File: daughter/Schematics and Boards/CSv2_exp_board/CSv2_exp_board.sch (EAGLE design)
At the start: 144 parts, among them J1 HIROSE-DF40_44-PIN_CONNECTORS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, J2 J-SERIAL-PORT, J3 CORTEX_DEBUG_SMD, J4 SJ-43514-SMT, J5 HIROSE-DF40_44-PIN_CONNECTORS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, J6 ATTINY_AVR_DEBUG, J7 J-USB-HIROSE-MICRO-USB, SW1 SPST_TACT-KMR2, SW2 SPST_TACT-KMR2, T1 TPTP10SQ, T10 TPTP10SQ, T11 TPTP10SQ, T2 TPTP10SQ, T3 TPTP10SQ, T4 TPTP10SQ, T5 TPTP10SQ, T6 TPTP10SQ, T7 TPTP10SQ, T8 TPTP10SQ, T9 TPTP10SQ, U1 LOADSWITCH-MIC94164, U10 LOADSWITCH-MIC94164, U11 BMI160, U12 TLV320DAC26IRHB, U13 ADG839YKSZ-500RL7KS_6_ADI-L, U14 LOADSWITCH-MIC94164, U15 LP2980AIM5-2.5/NOPBMF05A_TEX-L, U16 NCP553SQ18T1GSC-82AB_ONS-L, U17 ATTINY817-MFRQFN24_RX4MC-L_AT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, U18 MPL3115A2, U19 ATSAMD21G18_QFN, U2 ADA4841-1YRJZ-R7RJ_6-L, U3 Value, U4 RFM69HCW, U5 Value, U6 Value, U7 LOADSWITCH-MIC94164, U8 LOADSWITCH-MIC94164, U9 LOADSWITCH-MIC94164, X1 32.768kHz, X2 32.768, X3 uFL, X4 uFL, X5 uFL, X6 uFL

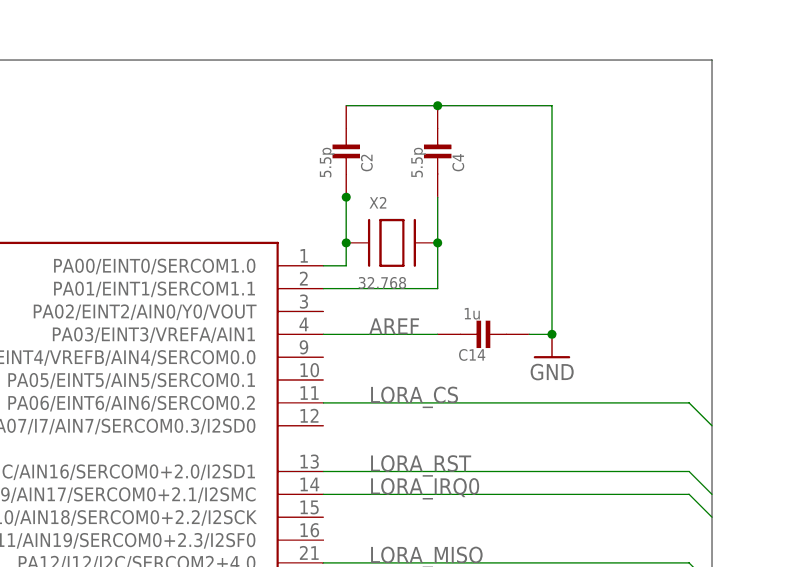
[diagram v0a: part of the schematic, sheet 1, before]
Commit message: DTR-filled in device attributes
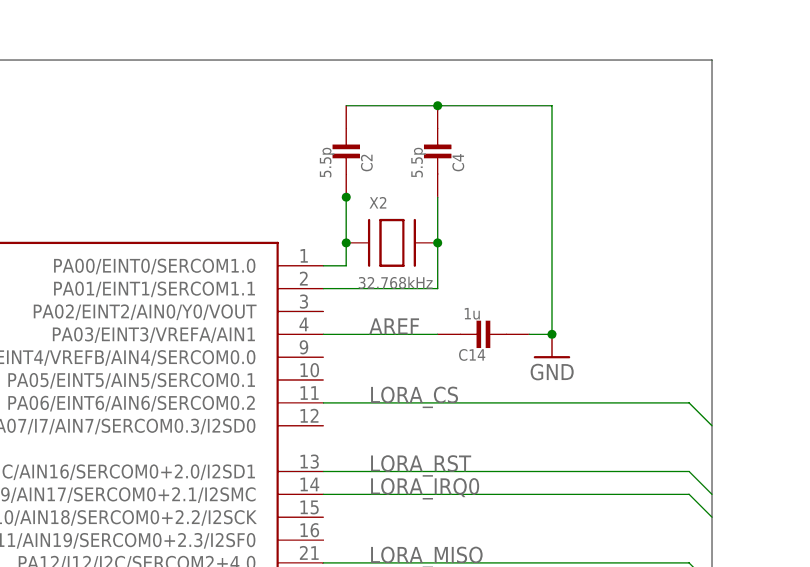
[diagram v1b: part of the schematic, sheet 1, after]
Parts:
- X2: value 32.768 -> 32.768kHz; DESC (none) -> CRYSTAL 32.7680KHZ 6PF SMD; HEIGHT (none) -> 0.9mm; LOAD_CAPACITY 6p -> 6pF; SIZE (none) -> 0.126" L x 0.059" W (3.20mm x 1.50mm); TOL (none) -> ±20ppm; TYPE (none) -> Crystal
- X3, X5, X6: DESC (none) -> CONN U.FL RCPT STR 50 OHM SMD; HEIGHT d -> 1.25mm; MANUFACTURER (none) -> Hirose; SIZE (none) -> 3.1 x 3mm; TYPE (none) -> Connector
- X4: DESC (none) -> CONN U.FL RCPT STR 50 OHM SMD; HEIGHT (none) -> 1.25mm; MEANUFACTURER (none) -> Hirose; SIZE (none) -> 3.1 x 3mm; TYPE (none) -> Connector
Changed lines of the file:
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@@
 <attribute name="Z-HEIGHT" value="0.55mm"/>
 </part>
-<part name="X2" library="CommonSense-DTR-v1" deviceset="ADAFRUIT2_XTAL" device="-3.2X1.5" value="32.768">
-<attribute name="DESC" value=""/>
-<attribute name="LOAD_CAPACITY" value="6p"/>
+<part name="X2" library="CommonSense-DTR-v1" deviceset="ADAFRUIT2_XTAL" device="-3.2X1.5" value="32.768kHz">
+<attribute name="DESC" value="CRYSTAL 32.7680KHZ 6PF SMD"/>
+<attribute name="HEIGHT" value="0.9mm"/>
+<attribute name="LOAD_CAPACITY" value="6pF"/>
 <attribute name="MANUFACTURER" value="NDK"/>
 <attribute name="MPN" value="NX3215SA-32.768K-STD-MUA-14"/>
 <attribute name="PARTNO" value="NX3215SA-32.768K-STD-MUA-14"/>
-<attribute name="SIZE" value=""/>
-<attribute name="TOL" value=""/>
-<attribute name="TYPE" value=""/>
-<attribute name="VOLT" value=""/>
+<attribute name="SIZE" value="0.126&quot; L x 0.059&quot; W (3.20mm x 1.50mm)"/>
+<attribute name="TOL" value="±20ppm"/>
+<attribute name="TYPE" value="Crystal"/>
 </part>
 <part name="U$14" library="Supplies" deviceset="GND" device=""/>
@@
 <part name="U$17" library="Supplies" deviceset="GND" device=""/>
 <part name="X4" library="Connectors" deviceset="J-U.FL" device="" value="uFL">
-<attribute name="DESC" value=""/>
+<attribute name="DESC" value="CONN U.FL RCPT STR 50 OHM SMD"/>
+<attribute name="HEIGHT" value="1.25mm"/>
+<attribute name="MEANUFACTURER" value="Hirose"/>
 <attribute name="MPN" value="U.FL-R-SMT-1(01)"/>
 <attribute name="PARTNO" value="U.FL-R-SMT-1(01)"/>
-<attribute name="SIZE" value=""/>
-<attribute name="TOL" value=""/>
-<attribute name="TYPE" value=""/>
-<attribute name="VOLT" value=""/>
+<attribute name="SIZE" value="3.1 x 3mm"/>
+<attribute name="TYPE" value="Connector"/>
 </part>
 <part name="U$23" library="Supplies" deviceset="GND" device=""/>
@@
 </part>
 <part name="X3" library="Connectors" deviceset="J-U.FL" device="" value="uFL">
-<attribute name="HEIGHT" value="d"/>
+<attribute name="DESC" value="CONN U.FL RCPT STR 50 OHM SMD"/>
+<attribute name="HEIGHT" value="1.25mm"/>
+<attribute name="MANUFACTURER" value="Hirose"/>
 <attribute name="MPN" value="U.FL-R-SMT-1(01)"/>
 <attribute name="PARTNO" value="U.FL-R-SMT-1(01)"/>
+<attribute name="SIZE" value="3.1 x 3mm"/>
+<attribute name="TYPE" value="Connector"/>
 </part>
 <part name="X5" library="Connectors" deviceset="J-U.FL" device="" value="uFL">
-<attribute name="HEIGHT" value="d"/>
+<attribute name="DESC" value="CONN U.FL RCPT STR 50 OHM SMD"/>
+<attribute name="HEIGHT" value="1.25mm"/>
+<attribute name="MANUFACTURER" value="Hirose"/>
 <attribute name="MPN" value="U.FL-R-SMT-1(01)"/>
 <attribute name="PARTNO" value="U.FL-R-SMT-1(01)"/>
+<attribute name="SIZE" value="3.1 x 3mm"/>
+<attribute name="TYPE" value="Connector"/>
 </part>
 <part name="X6" library="Connectors" deviceset="J-U.FL" device="" value="uFL">
-<attribute name="HEIGHT" value="d"/>
+<attribute name="DESC" value="CONN U.FL RCPT STR 50 OHM SMD"/>
+<attribute name="HEIGHT" value="1.25mm"/>
+<attribute name="MANUFACTURER" value="Hirose"/>
 <attribute name="MPN" value="U.FL-R-SMT-1(01)"/>
 <attribute name="PARTNO" value="U.FL-R-SMT-1(01)"/>
+<attribute name="SIZE" value="3.1 x 3mm"/>
+<attribute name="TYPE" value="Connector"/>
 </part>
 <part name="R7" library="Resistors" deviceset="R-" device="0402" value="50R">
@@
 <attribute name="TYPE" x="284.48" y="231.14" size="1.778" layer="96" display="off"/>
 <attribute name="SIZE" x="284.48" y="231.14" size="1.778" layer="96" display="off"/>
-<attribute name="VOLT" x="284.48" y="231.14" size="1.778" layer="96" display="off"/>
+<attribute name="HEIGHT" x="284.48" y="231.14" size="1.778" layer="96" display="off"/>
 </instance>
 <instance part="U$14" gate="1" x="101.6" y="233.68" smashed="yes">
@@
 <attribute name="MPN" x="78.62295625" y="212.957171875" size="1.778" layer="96" rot="R90" display="off"/>
 <attribute name="PARTNO" x="78.62295625" y="212.957171875" size="1.778" layer="96" display="off"/>
-<attribute name="TOL" x="78.62295625" y="212.957171875" size="1.778" layer="96" rot="R90" display="off"/>
 <attribute name="DESC" x="78.62295625" y="212.957171875" size="1.778" layer="96" rot="R90" display="off"/>
 <attribute name="TYPE" x="78.62295625" y="212.957171875" size="1.778" layer="96" rot="R90" display="off"/>
 <attribute name="SIZE" x="78.62295625" y="212.957171875" size="1.778" layer="96" rot="R90" display="off"/>
-<attribute name="VOLT" x="78.62295625" y="212.957171875" size="1.778" layer="96" rot="R90" display="off"/>
+<attribute name="HEIGHT" x="78.62295625" y="212.957171875" size="1.778" layer="96" rot="R90" display="off"/>
+<attribute name="MEANUFACTURER" x="78.62295625" y="212.957171875" size="1.778" layer="96" rot="R90" display="off"/>
 </instance>
 <instance part="U$23" gate="1" x="68.58" y="215.9" smashed="yes">
@@
 <attribute name="MPN" x="266.58295625" y="248.517171875" size="1.778" layer="96" rot="R90" display="off"/>
 <attribute name="PARTNO" x="266.58295625" y="248.517171875" size="1.778" layer="96" display="off"/>
+<attribute name="SIZE" x="266.58295625" y="248.517171875" size="1.778" layer="96" rot="R90" display="off"/>
+<attribute name="DESC" x="266.58295625" y="248.517171875" size="1.778" layer="96" rot="R90" display="off"/>
+<attribute name="TYPE" x="266.58295625" y="248.517171875" size="1.778" layer="96" rot="R90" display="off"/>
+<attribute name="MANUFACTURER" x="266.58295625" y="248.517171875" size="1.778" layer="96" rot="R90" display="off"/>
 <attribute name="HEIGHT" x="266.58295625" y="248.517171875" size="1.778" layer="96" rot="R90" display="off"/>
 </instance>
@@
 <attribute name="MPN" x="297.06295625" y="248.517171875" size="1.778" layer="96" rot="R90" display="off"/>
 <attribute name="PARTNO" x="297.06295625" y="248.517171875" size="1.778" layer="96" display="off"/>
+<attribute name="SIZE" x="297.06295625" y="248.517171875" size="1.778" layer="96" rot="R90" display="off"/>
+<attribute name="DESC" x="297.06295625" y="248.517171875" size="1.778" layer="96" rot="R90" display="off"/>
+<attribute name="TYPE" x="297.06295625" y="248.517171875" size="1.778" layer="96" rot="R90" display="off"/>
+<attribute name="MANUFACTURER" x="297.06295625" y="248.517171875" size="1.778" layer="96" rot="R90" display="off"/>
 <attribute name="HEIGHT" x="297.06295625" y="248.517171875" size="1.778" layer="96" rot="R90" display="off"/>
 </instance>
@@
 <attribute name="MPN" x="330.08295625" y="248.517171875" size="1.778" layer="96" rot="R90" display="off"/>
 <attribute name="PARTNO" x="330.08295625" y="248.517171875" size="1.778" layer="96" display="off"/>
+<attribute name="SIZE" x="330.08295625" y="248.517171875" size="1.778" layer="96" rot="R90" display="off"/>
+<attribute name="DESC" x="330.08295625" y="248.517171875" size="1.778" layer="96" rot="R90" display="off"/>
+<attribute name="TYPE" x="330.08295625" y="248.517171875" size="1.778" layer="96" rot="R90" display="off"/>
+<attribute name="MANUFACTURER" x="330.08295625" y="248.517171875" size="1.778" layer="96" rot="R90" display="off"/>
 <attribute name="HEIGHT" x="330.08295625" y="248.517171875" size="1.778" layer="96" rot="R90" display="off"/>
 </instance>
